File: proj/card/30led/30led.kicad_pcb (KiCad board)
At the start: 2 copper layers, 100 x 75 mm, 52 parts, among them J1 USB_C_Receptacle_USB2.0_16P, SW1 SW_Push, SW2 SW_Push, U1 ATtiny404-SS, U2 CH340K

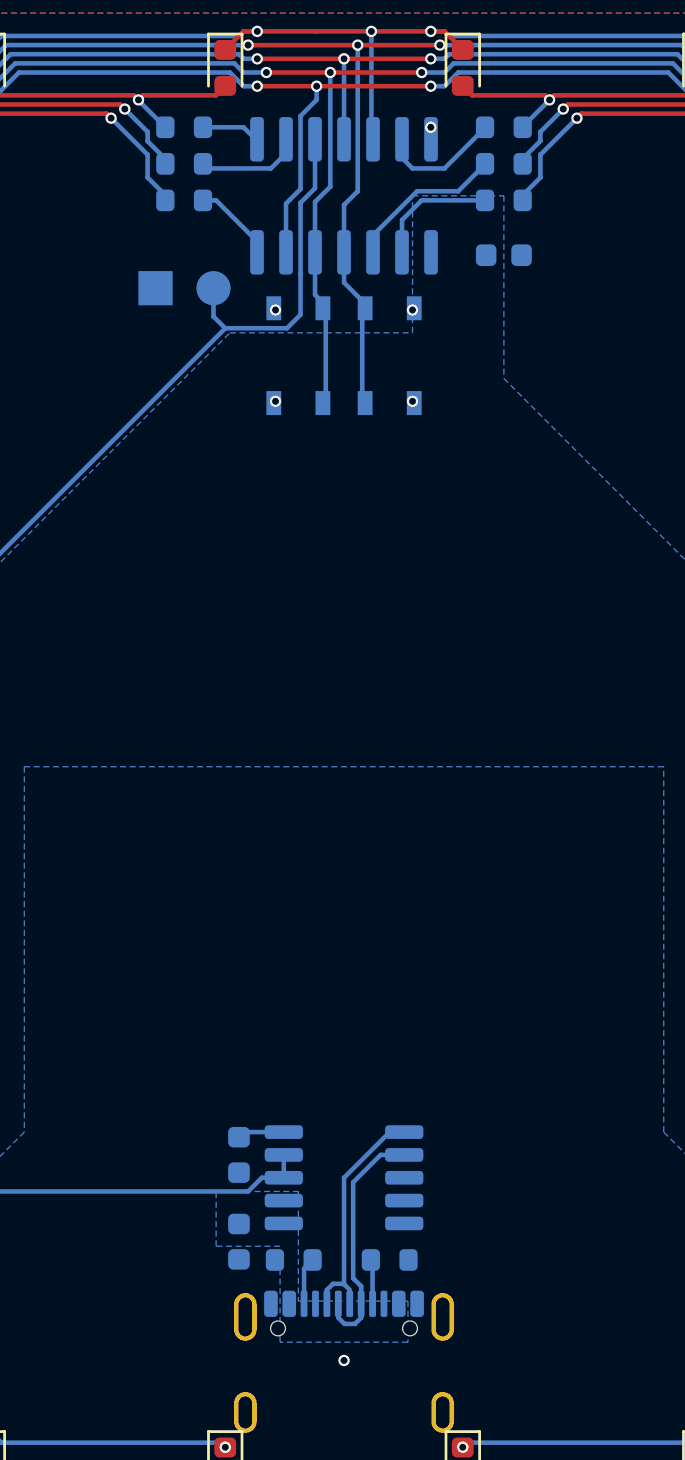
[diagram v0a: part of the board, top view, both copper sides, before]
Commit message: -
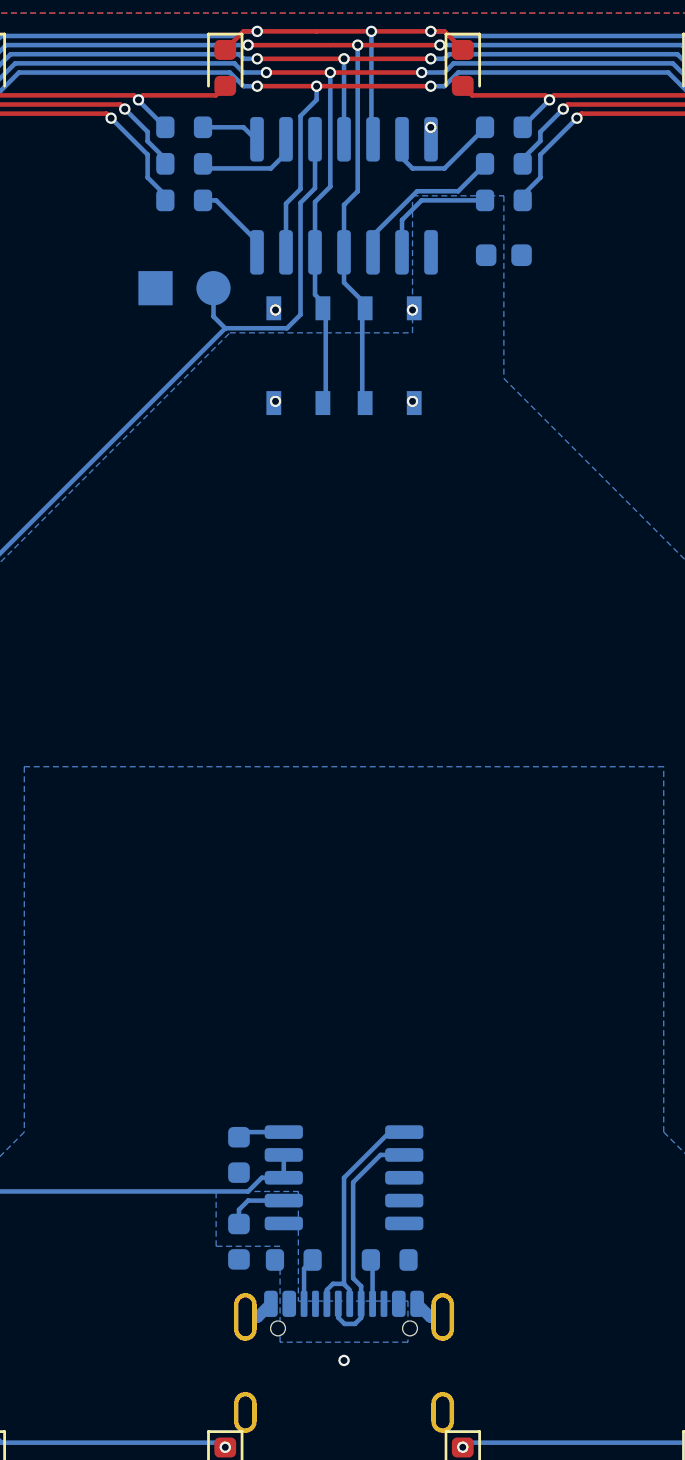
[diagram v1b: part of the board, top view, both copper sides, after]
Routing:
- net VBUS: track 0.00 -> 2.75 mm
- net GND: track 0.00 -> 2.72 mm
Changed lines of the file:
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@@
 	)
 	(segment
+		(start 103.775 124.095)
+		(end 103.2 123.52)
+		(width 0.5)
+		(layer "B.Cu")
+		(net 1)
+	)
+	(segment
+		(start 104.32 124.095)
+		(end 103.775 124.095)
+		(width 0.5)
+		(layer "B.Cu")
+		(net 1)
+	)
+	(segment
+		(start 95.68 124.095)
+		(end 96.225 124.095)
+		(width 0.5)
+		(layer "B.Cu")
+		(net 1)
+	)
+	(segment
+		(start 96.225 124.095)
+		(end 96.8 123.52)
+		(width 0.5)
+		(layer "B.Cu")
+		(net 1)
+	)
+	(segment
 		(start 102.54 76.06)
 		(end 102.54 77.475)
@@
 	)
 	(segment
-		(start 98.73 74.67)
-		(end 98.095 75.305)
-		(width 0.2)
-		(layer "B.Cu")
-		(net 12)
-	)
-	(segment
 		(start 65.8 126.2)
 		(end 59.8 120.2)
@@
 	)
 	(segment
-		(start 97.502 80.8)
-		(end 98.095 80.207)
+		(start 83.8 118.6)
+		(end 76.2 126.2)
 		(width 0.2)
 		(layer "B.Cu")
@@
 	)
 	(segment
-		(start 83.8 118.6)
-		(end 76.2 126.2)
+		(start 97.502 80.8)
+		(end 98.095 80.207)
 		(width 0.2)
 		(layer "B.Cu")
@@
 	)
 	(segment
-		(start 98.095 80.207)
-		(end 98.095 78.4)
+		(start 97.3625 118)
+		(end 96.4 118)
 		(width 0.2)
 		(layer "B.Cu")
@@
 	)
 	(segment
-		(start 97.3625 118)
-		(end 96.4 118)
+		(start 81.8 93.8)
+		(end 94.8 80.8)
 		(width 0.2)
 		(layer "B.Cu")
@@
 	)
 	(segment
-		(start 98.095 78.4)
-		(end 98.095 78.456968)
+		(start 94.8 80.8)
+		(end 97.502 80.8)
 		(width 0.2)
 		(layer "B.Cu")
@@
 	)
 	(segment
-		(start 81.8 93.8)
-		(end 94.8 80.8)
+		(start 98.095 80.207)
+		(end 98.095 75.305)
 		(width 0.2)
 		(layer "B.Cu")
@@
 	)
 	(segment
-		(start 98.095 75.305)
-		(end 98.095 78.4)
+		(start 96.4 118)
+		(end 95.8 118.6)
 		(width 0.2)
 		(layer "B.Cu")
@@
 	)
 	(segment
-		(start 94.8 80.8)
-		(end 97.502 80.8)
+		(start 98.73 74.67)
+		(end 98.73 72.525)
 		(width 0.2)
 		(layer "B.Cu")
@@
 	)
 	(segment
-		(start 96.4 118)
-		(end 95.8 118.6)
+		(start 98.095 75.305)
+		(end 98.73 74.67)
 		(width 0.2)
 		(layer "B.Cu")
@@
 	)
 	(segment
-		(start 98.73 72.525)
-		(end 98.73 74.67)
-		(width 0.2)
-		(layer "B.Cu")
-		(net 12)
-	)
-	(segment
 		(start 94.285 79.045)
 		(end 94.285 80.285)
@@
 	)
 	(segment
+		(start 95.8 119)
+		(end 97.3625 119)
+		(width 0.2)
+		(layer "B.Cu")
+		(net 22)
+	)
+	(segment
+		(start 95.4 119.4)
+		(end 95.8 119)
+		(width 0.2)
+		(layer "B.Cu")
+		(net 22)
+	)
+	(segment
+		(start 95.4 120.025)
+		(end 95.4 119.4)
+		(width 0.2)
+		(layer "B.Cu")
+		(net 22)
+	)
+	(segment
